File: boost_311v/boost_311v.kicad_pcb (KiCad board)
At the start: 2 copper layers, 59 parts, among them J1 Vin_cnt, J2 VO, J3 Vin_boost, Q1 BC556, Q2 PN2222A, Q3 PN2222A, Q4 PN2222A, Q5 IRFP260, Q6 2N3904, Q7 2N3906, U2 L7812, U3 4N25, U4 LF357, U5 NE555

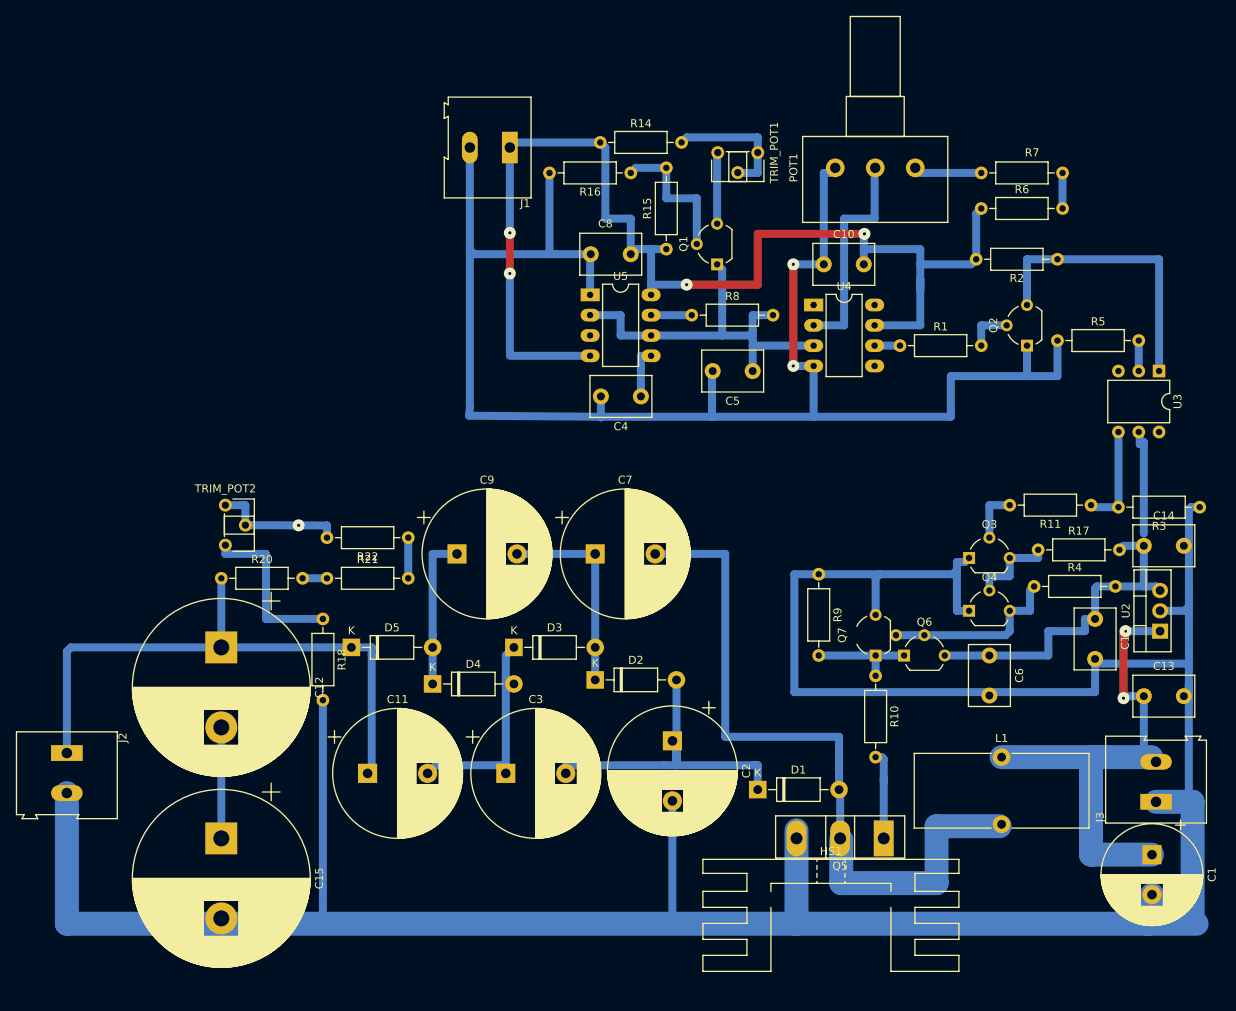
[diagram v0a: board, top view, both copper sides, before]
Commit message: Up pcbs
Signed-off-by: fgl27 <fglfgl27@gmail.com>
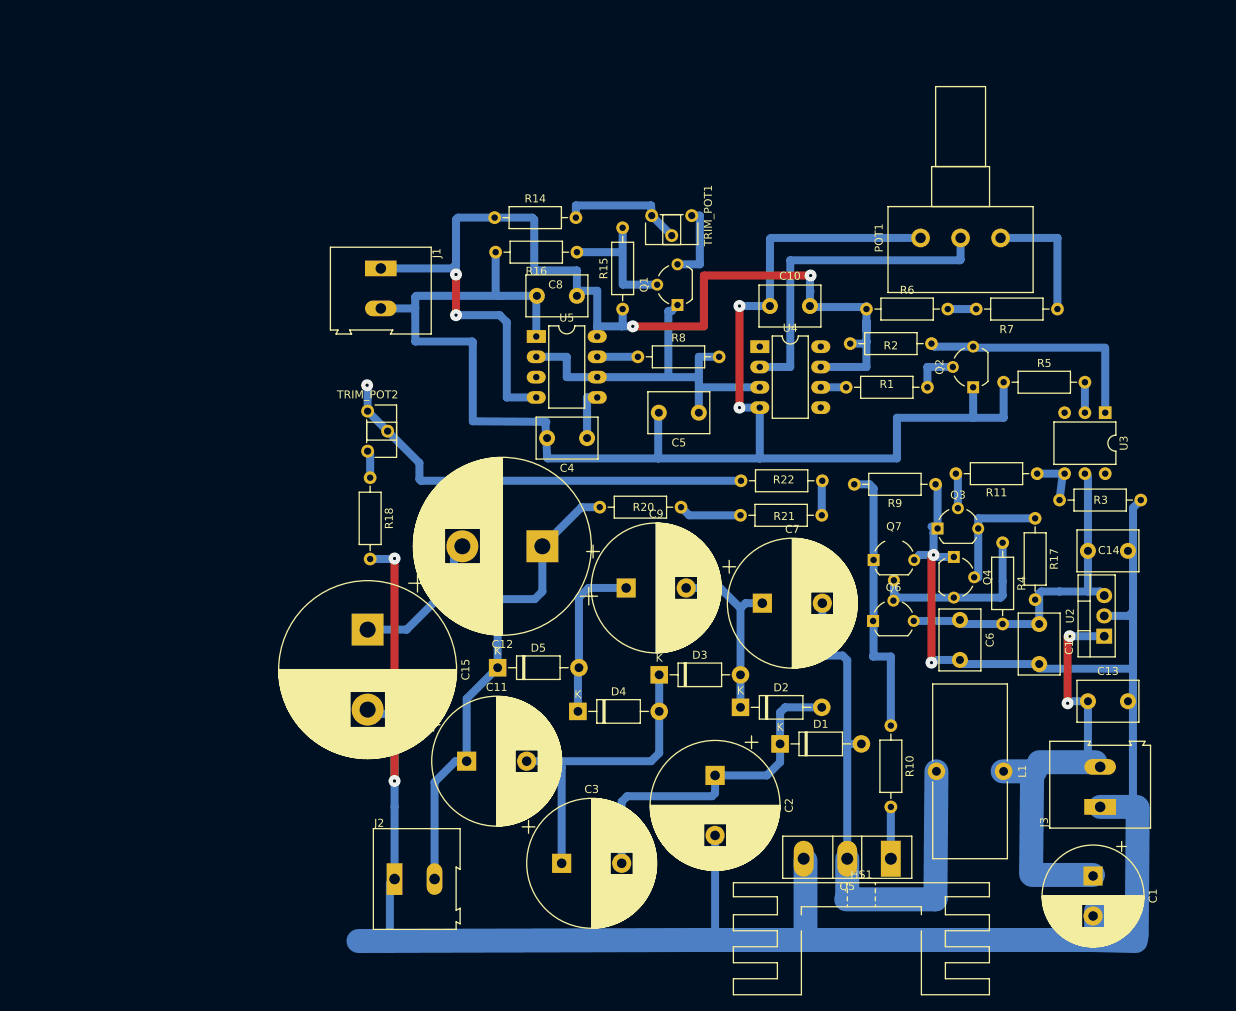
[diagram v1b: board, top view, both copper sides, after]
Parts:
- moved R21 52.3 mm to (116.7, 129.8)
- moved R22 52.2 mm to (126.9, 125.5)
- moved R20 48.1 mm to (99.1, 128.8)
- moved J2 43.9 mm to (73.5, 175.3), turned to 0 degrees
- moved C12 42.1 mm to (91.9, 133.7), turned to 180 degrees
- moved C15 31.9 mm to (70.1, 144.1)
- moved J1 22.1 mm to (71.8, 98.9), turned to 270 degrees
- moved C7 21.8 mm to (119.4, 140.8)
- moved C9 21.6 mm to (102.4, 138.9)
- moved TRIM_POT2 21.3 mm to (70.1, 116.8)
- moved R7 20.2 mm to (146.2, 104.0), turned to 0 degrees
- moved R6 19.1 mm to (132.5, 104.0)
- moved R2 19.0 mm to (140.6, 108.3)
- moved R18 18.6 mm to (70.4, 125.1)
- moved D3 18.5 mm to (106.6, 149.7)
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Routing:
- net GND2: track 385.3 -> 308.6 mm, vias 0 -> 4
- net /10%_VO: track 16.7 -> 54.7 mm
- net Net-(C7-Pad2): track 91.5 -> 69.6 mm
- net /MOS_Gate: track 13.2 -> 34.5 mm
- net Net-(R18-Pad1): track 21.4 -> 3.45 mm
- net Net-(C11-Pad1): track 74.9 -> 60.0 mm
- net /12V_L7812: track 57.5 -> 42.9 mm
- net Net-(C11-Pad2): track 25.9 -> 40.4 mm
- net Net-(POT1-Pad2): track 27.3 -> 41.2 mm
- net +12V: track 149.4 -> 137.7 mm
- net Net-(POT1-Pad1): track 8.52 -> 16.0 mm
- net +24V: track 66.0 -> 58.6 mm
- net Net-(Q5-Pad1): track 11.5 -> 5.08 mm
- net Net-(R11-Pad1): track 12.9 -> 6.50 mm
- net /PWM: track 36.2 -> 30.0 mm
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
